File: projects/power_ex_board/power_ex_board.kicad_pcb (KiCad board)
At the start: 2 copper layers, 34.6 x 26.4 mm, 19 parts, among them J1 USB_C_Receptacle_USB2.0, J2 3V3, J3 GND, J4 5V, J5 GND, J6 Custom, J7 GND, U1 ETA3409S2F

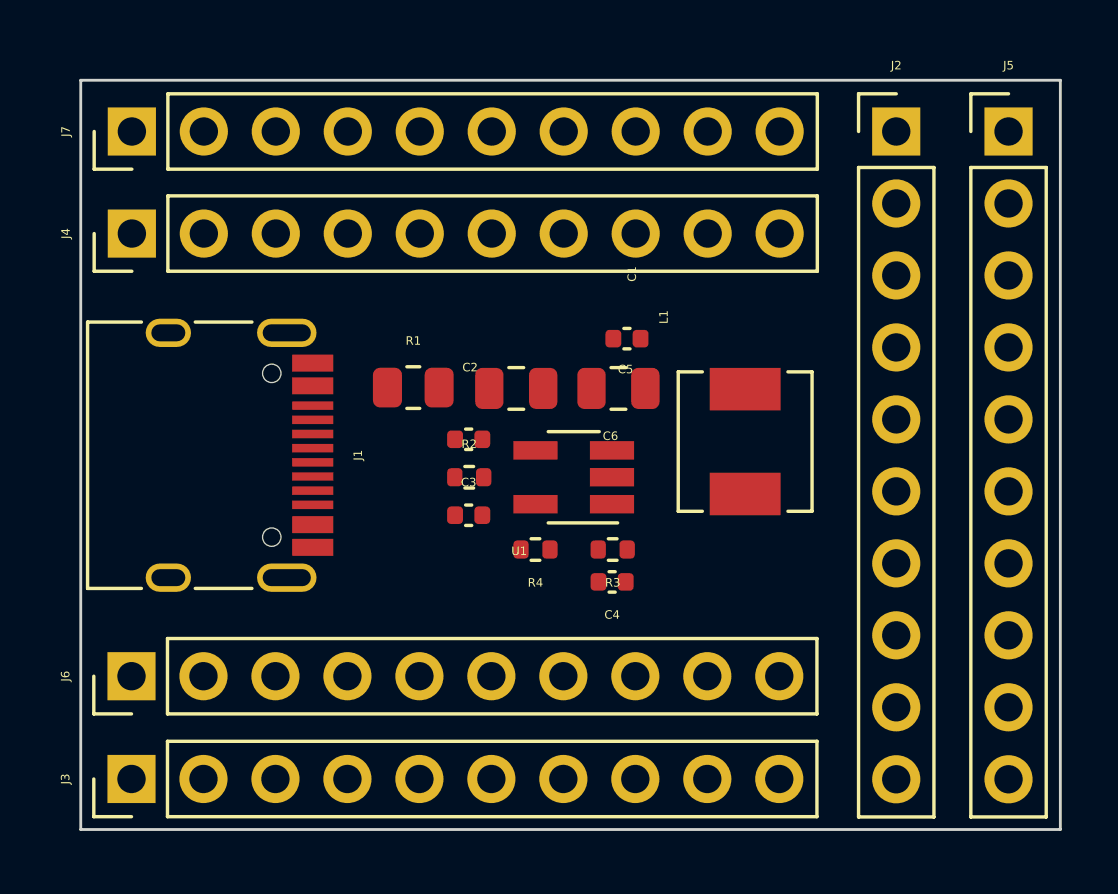
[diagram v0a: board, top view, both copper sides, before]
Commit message: projects: add power_ex_board
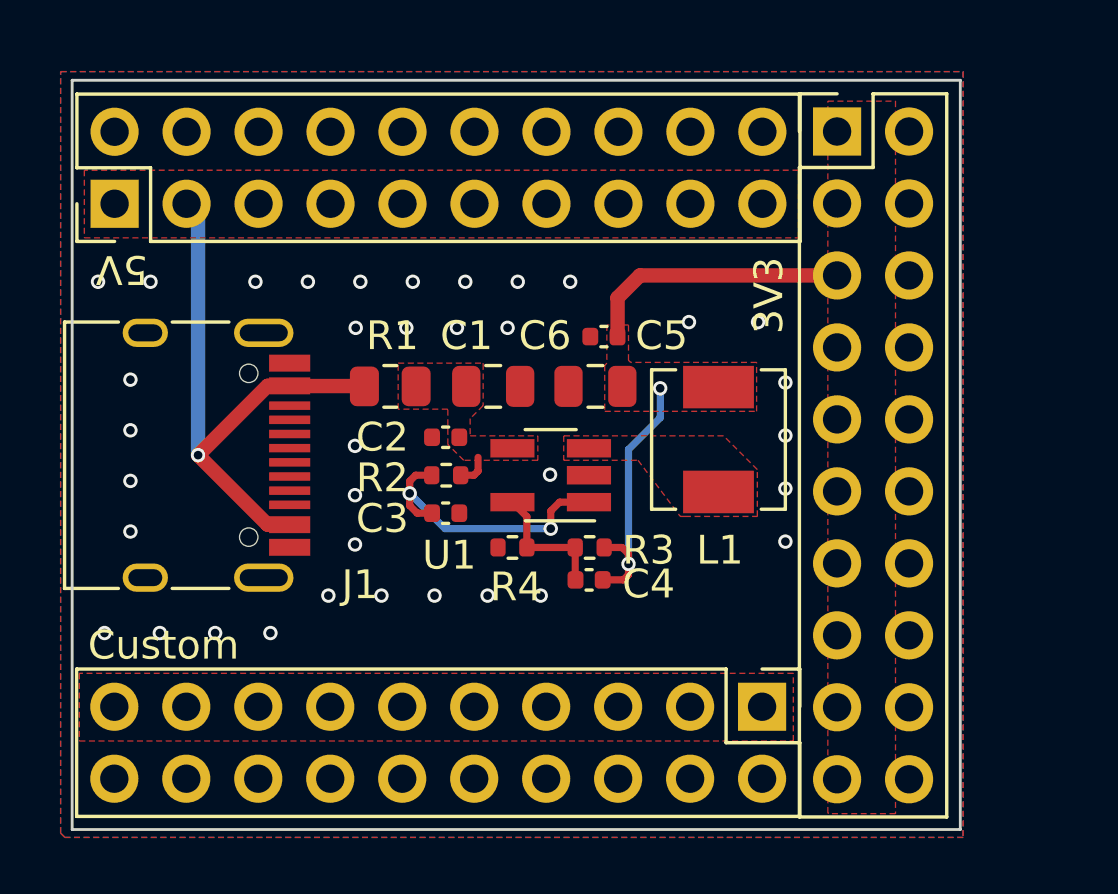
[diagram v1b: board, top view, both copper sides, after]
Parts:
- removed J2: 3V3, Connector_PinHeader_2.54mm:PinHeader_1x10_P2.54mm_Vertical
- removed J3, J5, J7: GND, Connector_PinHeader_2.54mm:PinHeader_1x10_P2.54mm_Vertical
- removed J4: 5V, Connector_PinHeader_2.54mm:PinHeader_1x10_P2.54mm_Vertical
- removed J6: Custom, Connector_PinHeader_2.54mm:PinHeader_1x10_P2.54mm_Vertical
- added 3V3: 3V3, Connector_PinHeader_2.54mm:PinHeader_2x10_P2.54mm_Vertical, F.Cu at (119.1, 97.5)
- added 5V: 5V, Connector_PinHeader_2.54mm:PinHeader_2x10_P2.54mm_Vertical, F.Cu at (93.6, 100.1)
- added Custom: Custom, Connector_PinHeader_2.54mm:PinHeader_2x10_P2.54mm_Vertical, F.Cu at (116.5, 117.8)
- moved L1 0.94 mm to (114.9, 108.4)
- moved C5 0.82 mm to (110.9, 104.8)
- moved C6 0.82 mm to (110.6, 106.5)
- moved R4 0.82 mm to (107.7, 112.2)
- moved C1 0.82 mm to (107.0, 106.5)
- moved C2 0.82 mm to (105.3, 108.3)
- moved C3 0.82 mm to (105.3, 111.0)
- moved C4 0.82 mm to (110.4, 113.4)
- moved R2 0.82 mm to (105.3, 109.7)
- moved R3 0.82 mm to (110.4, 112.2)
- moved U1 0.82 mm to (109.0, 109.7)
- moved R1 0.81 mm to (103.4, 106.5)
- moved J1 0.81 mm to (95.8, 109.0)
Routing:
- net +5V: track 0.00 -> 20.2 mm, vias 0 -> 1
- net +3V3: track 0.00 -> 18.8 mm, vias 0 -> 2
- net Net-(U1-EN): track 0.00 -> 10.2 mm, vias 0 -> 2
- net Net-(U1-FB): track 0.00 -> 4.66 mm
- net Net-(U1-IN): track 0.00 -> 1.16 mm
- net GND: vias 0 -> 36
- added copper zone on F.Cu, net +3V3
- added copper zone on F.Cu, net +5V
- added copper zone on B.Cu, net GND
- added copper zone on F.Cu, net GND
- added copper zone on F.Cu, net Net-(U1-IN)
- added copper zone on F.Cu, net Net-(U1-LX)
- added copper zone on F.Cu, net VCC
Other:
- board size 34.6 x 26.4 mm -> 31.3 x 26.4 mm
- board text added: "ESP-Power-Ex-Board"
